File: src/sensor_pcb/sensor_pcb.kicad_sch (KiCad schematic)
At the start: 18 parts, among them IC1 TCAN3414DRBR, J1 643280100305, J2 643280100305, J3 66200821022, J4 66200821022, U1 SHT45-AD1B, U2 16-bit ADC, U4 BMP581

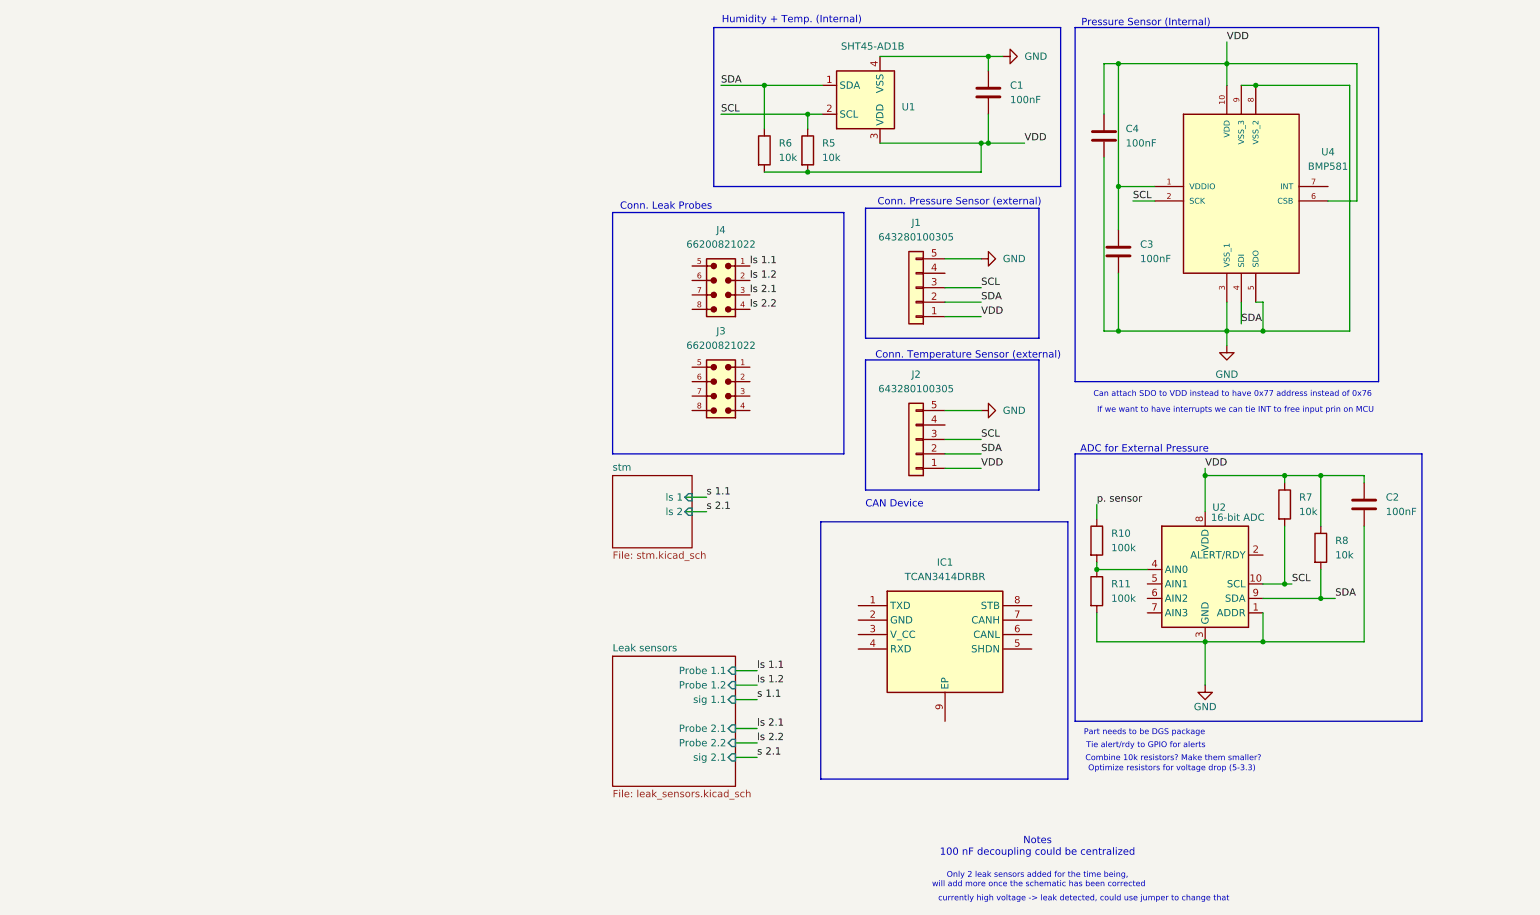
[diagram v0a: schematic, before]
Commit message: v1 complete
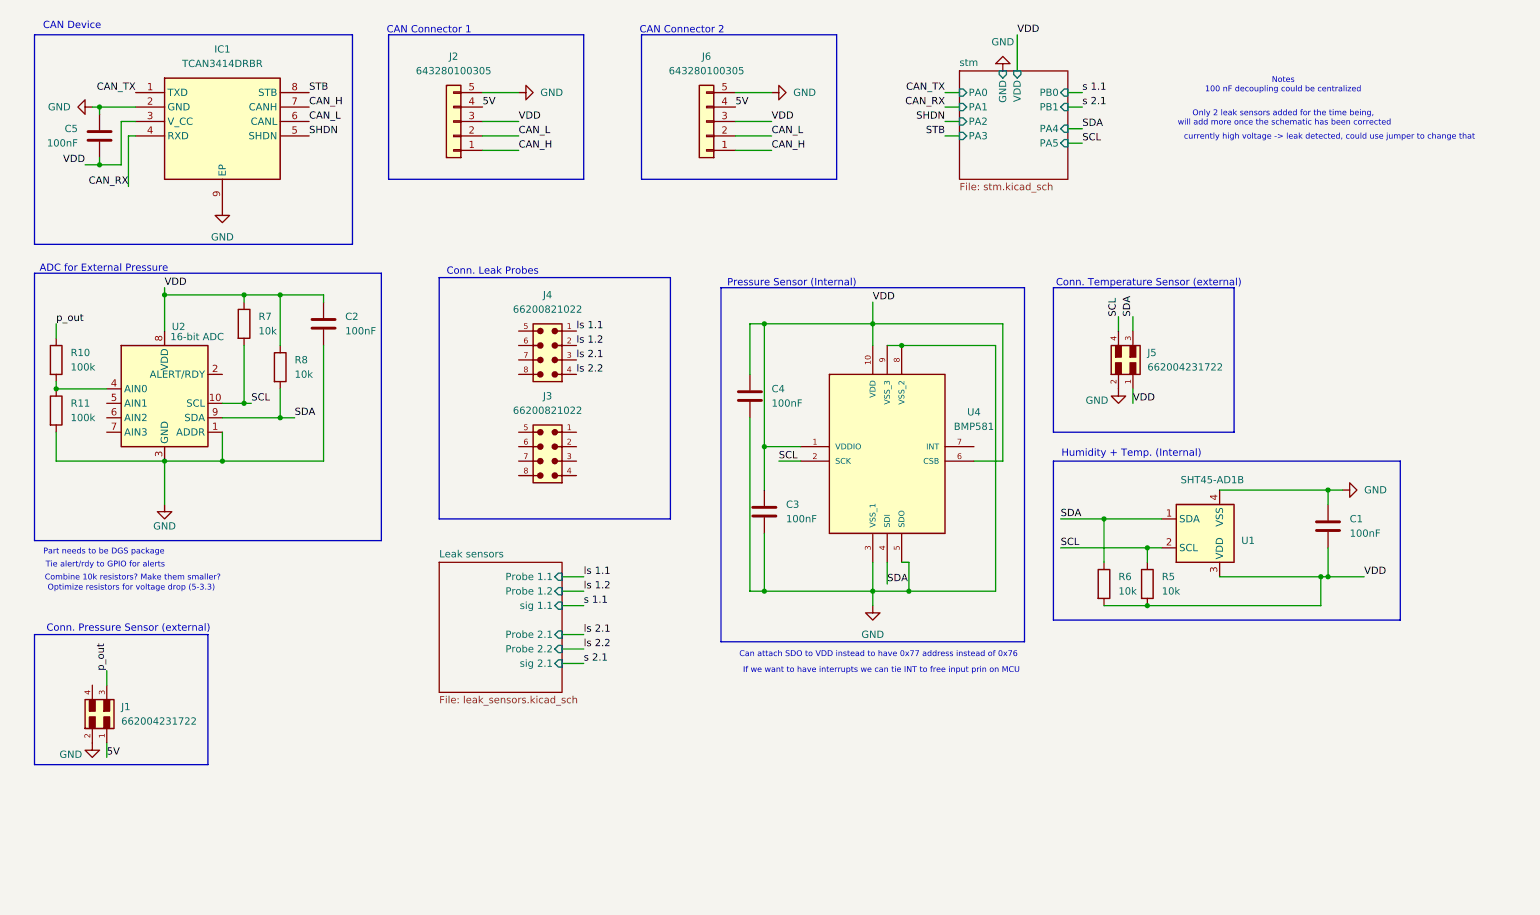
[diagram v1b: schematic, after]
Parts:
- removed J1: 643280100305, dz_con:Wuerth_WR_CIRCM_643280100305, symbol #dzdb:s_con/CON-WUR-643280100305
- added C5: 100nF, Capacitor_SMD:C_0402_1005Metric, symbol #dzdb:g_cap/C-100n-0402
- added J1, J5: 662004231722, dz_con:Wurth_662004231722, symbol #dzdb:s_con/CON-WUR-662004231722
- added J6: 643280100305, dz_con:Wuerth_WR_CIRCM_643280100305, symbol #dzdb:s_con/CON-WUR-643280100305
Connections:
- net GND: now also IC1.2 (GND), IC1.9 (EP), C5.1, J1.2, J5.2, J6.5 (Pin_5)
- net SCL: now also J5.4; no longer J2.3 (Pin_3)
- net SDA: now also J5.3; no longer J2.2 (Pin_2)
- net VDD: now also IC1.3 (V_CC), J2.3 (Pin_3), C5.2, J5.1, J6.3 (Pin_3); no longer J2.1 (Pin_1)
- net CAN_TX: now reaches IC1.1 (TXD)
- net CAN_RX: now reaches IC1.4 (RXD)
- net SHDN: now reaches IC1.5 (SHDN)
- net CAN_L: now reaches IC1.6 (CANL)
- net CAN_L: now also J2.2 (Pin_2), J6.2 (Pin_2)
- net CAN_H: now reaches IC1.7 (CANH)
- net CAN_H: now also J2.1 (Pin_1), J6.1 (Pin_1)
- net STB: now reaches IC1.8 (STB)
- net 5V: now reaches J2.4 (Pin_4)
- net 5V: now also J1.1, J6.4 (Pin_4)
- net p. sensor renamed p_out
- net p_out: now also J1.3
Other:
- sheet stm ports: added GND, PA0, PA1, PA2, PA3, PA4, PA5, PB0, PB1, VDD; removed ls 1, ls 2
- note added: "CAN Connector 1"
- note added: "CAN Connector 2"
- company: (none) -> Giacomo Raggi
- title: (none) -> Sensor PCB
- moved on the sheet: C1, C2, C3, C4, IC1, J3, J4, R10, R11, R5, R6, R7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
